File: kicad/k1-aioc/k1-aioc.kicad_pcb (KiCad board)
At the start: 2 copper layers, 21 x 31.5 mm, 45 parts, among them J1 12401832E402A, J2 Conn_01x07_Male, Q1 BC847BS, U1 MIC5330-SSYML, U2 STM32F373CBTx, Y1 8MHz/20pF

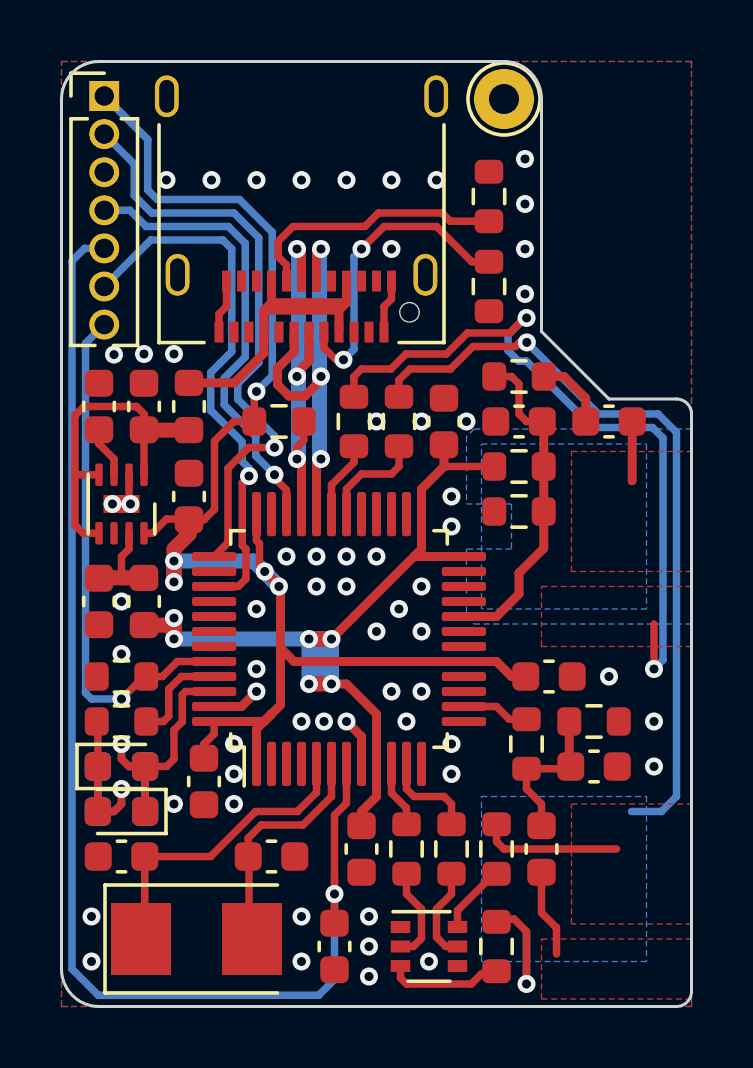
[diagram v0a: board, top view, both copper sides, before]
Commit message: Added additional attenuation functionality for DAC
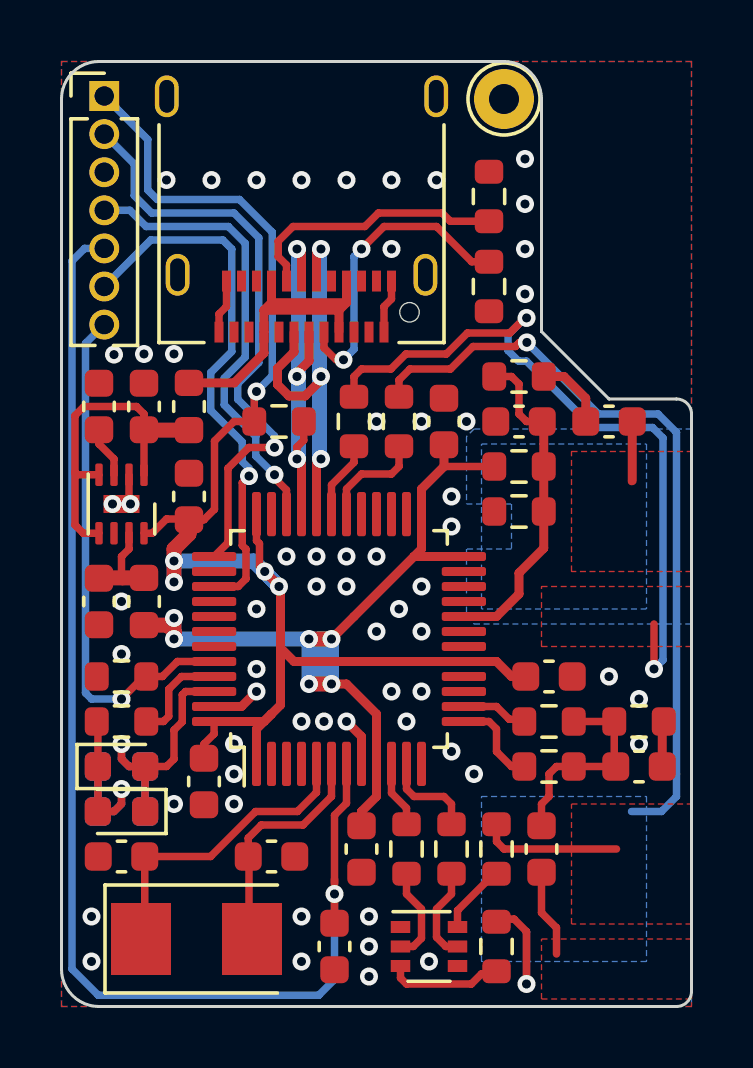
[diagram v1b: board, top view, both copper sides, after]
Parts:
- added R17: 220R, Resistor_SMD:R_0603_1608Metric, F.Cu at (119.8, 103.5)
- moved C12 1.50 mm to (122.8, 103.5)
- moved R4 1.50 mm to (122.8, 102.0)
- moved R2 1.06 mm to (119.8, 102.0), turned to 0 degrees
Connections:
- U2 pad 13: unconnected-(U2-Pad13) -> /GPIO-OD
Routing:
- net /GPIO-OD: track 0.00 -> 3.07 mm
- net Net-(C12-Pad1): track 5.13 -> 7.03 mm
- net GND: track 7.84 -> 9.36 mm

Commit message: Changed R2 to 5.1K to decrease DAC loading and reduce output level for radio microphone input
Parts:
- R2: value 2.2K -> 5.1K
- turned R2 to 180 degrees
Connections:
- R2 pad 1: /AFOUT -> Net-(C12-Pad1)
- R2 pad 2: Net-(C12-Pad1) -> /AFOUT
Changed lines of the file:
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@@
   (net 60 "/GPIO-OD")
   (footprint "Resistor_SMD:R_0603_1608Metric" (layer "F.Cu")
-    (at 119.75 102)
+    (at 119.75 102 180)
     (descr "Resistor SMD 0603 (1608 Metric), square (rectangular) end terminal, IPC_7351 nominal, (Body size source: IPC-SM-782 page 72, https://www.pcb-3d.com/wordpress/wp-content/uploads/ipc-sm-782a_amendment_1_and_2.pdf), generated with kicad-footprint-generator")
     (tags "resistor")
-    (property "LCSC" "C4190")
+    (property "LCSC" "C23186")
     (property "Sheetfile" "File: k1-aioc.kicad_sch")
     (property "Sheetname" "")
@@
       (effects (font (size 0.5 0.5) (thickness 0.1)))
     )
-    (fp_text value "2.2K" (at 0 1.43) (layer "F.Fab")
+    (fp_text value "5.1K" (at 0 1.43) (layer "F.Fab")
       (effects (font (size 1 1) (thickness 0.15)))
     )
@@
     (fp_line (start -0.8 -0.4125) (end 0.8 -0.4125) (layer "F.Fab") (width 0.1))
     (fp_line (start 0.8 -0.4125) (end 0.8 0.4125) (layer "F.Fab") (width 0.1))
-    (pad "1" smd roundrect (at -0.825 0) (size 0.8 0.95) (layers "F.Cu" "F.Paste" "F.Mask") (roundrect_rratio 0.25)
+    (pad "1" smd roundrect (at -0.825 0 180) (size 0.8 0.95) (layers "F.Cu" "F.Paste" "F.Mask") (roundrect_rratio 0.25)
+      (net 32 "Net-(C12-Pad1)") (pintype "passive"))
+    (pad "2" smd roundrect (at 0.825 0 180) (size 0.8 0.95) (layers "F.Cu" "F.Paste" "F.Mask") (roundrect_rratio 0.25)
       (net 45 "/AFOUT") (pintype "passive"))
-    (pad "2" smd roundrect (at 0.825 0) (size 0.8 0.95) (layers "F.Cu" "F.Paste" "F.Mask") (roundrect_rratio 0.25)
-      (net 32 "Net-(C12-Pad1)") (pintype "passive"))
     (model "${KICAD6_3DMODEL_DIR}/Resistor_SMD.3dshapes/R_0603_1608Metric.wrl"
       (offset (xyz 0 0 0))
